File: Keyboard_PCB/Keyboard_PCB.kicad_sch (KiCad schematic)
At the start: 59 parts, among them J2 Battery, J3 JTAG, J4 EBUS, SW71 BTN, SW72 BTN, U1 STM32H7B0VBTx, U3 AP7343, U4 M95P32, Y1 25MHz, Y2 32.768 KHz

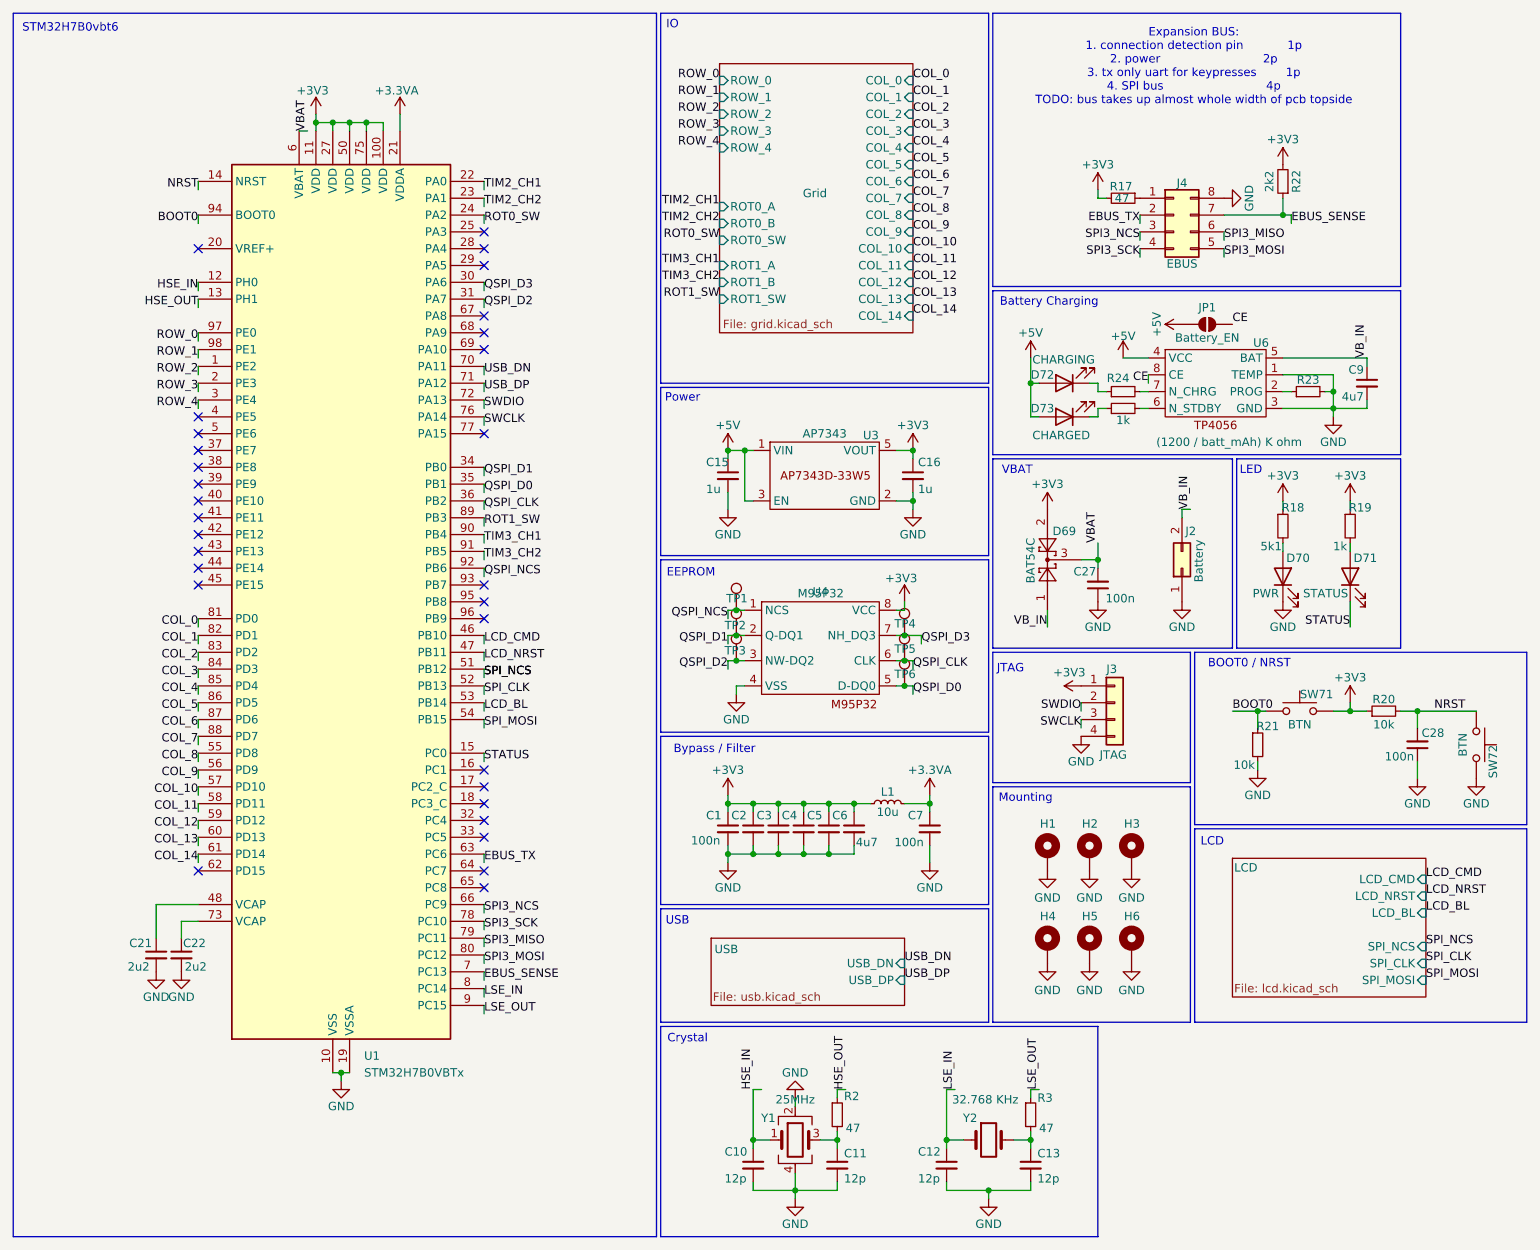
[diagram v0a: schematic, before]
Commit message: Cleaned up project
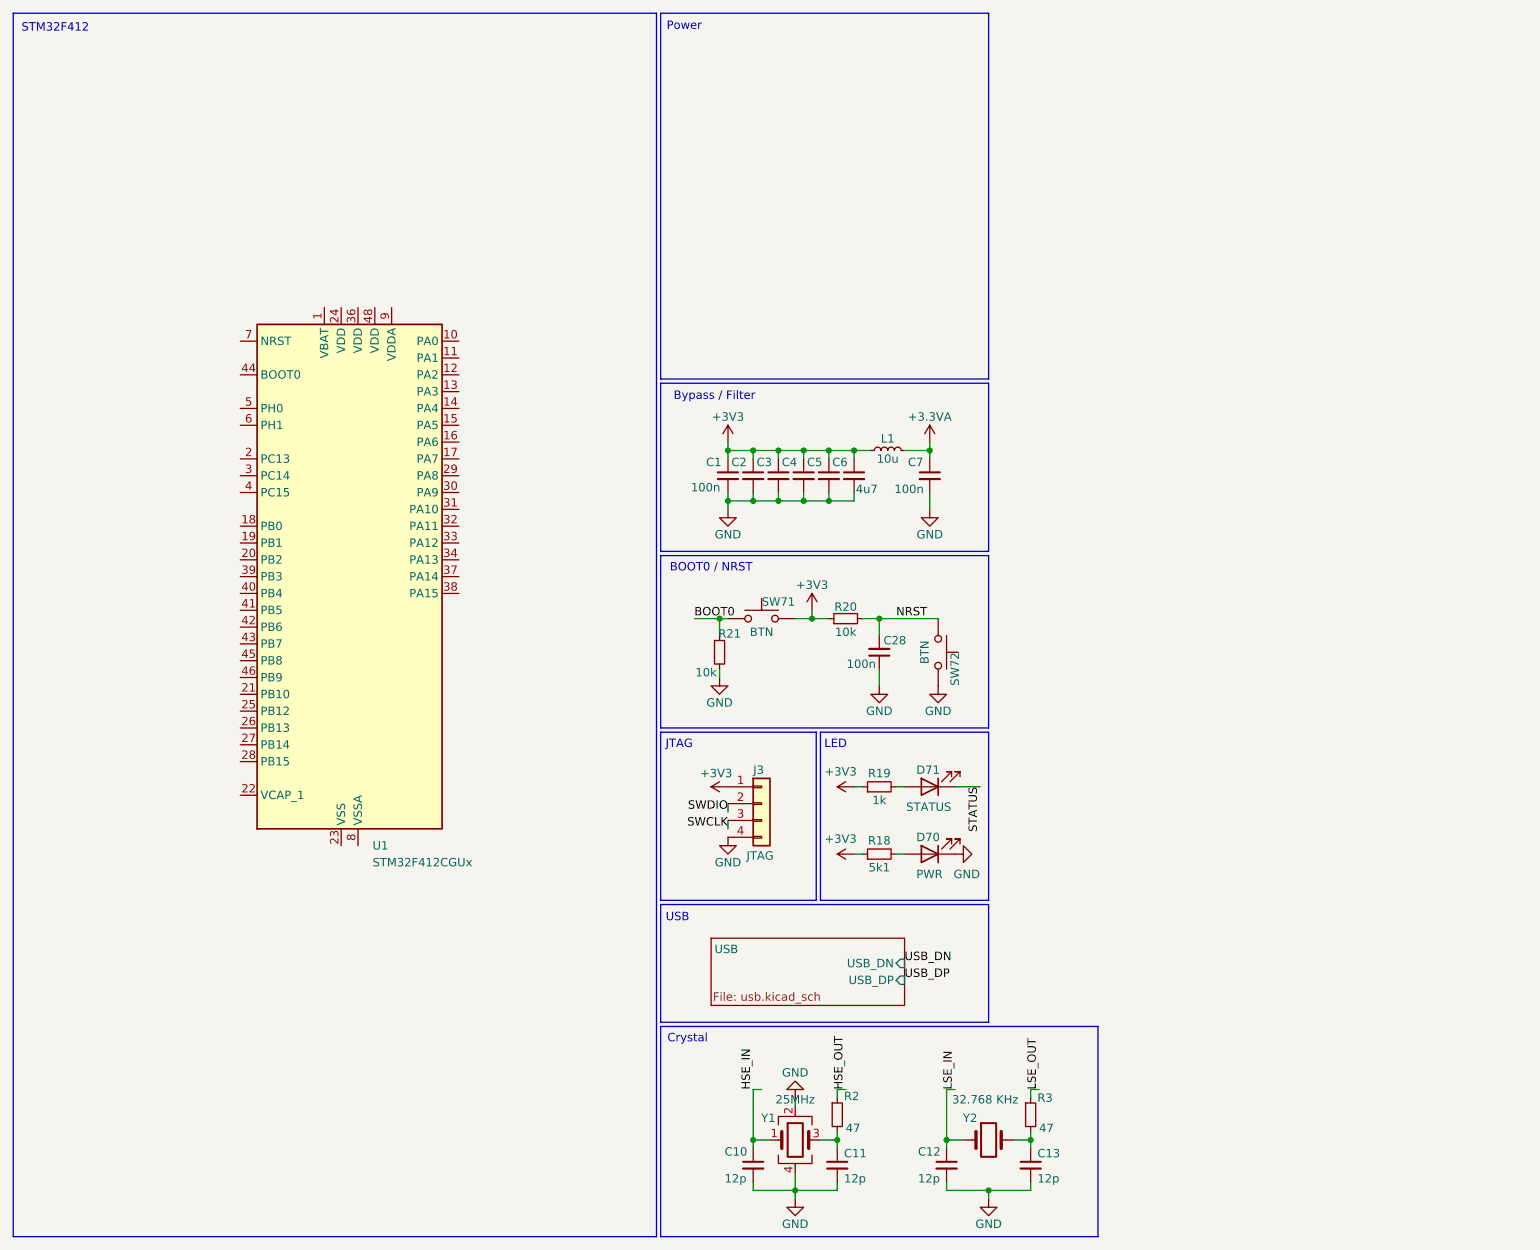
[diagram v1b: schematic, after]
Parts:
- removed C15, C16: 1u, Capacitor_SMD:C_0603_1608Metric, symbol Device:C_Small
- removed C21, C22: 2u2, Capacitor_SMD:C_0603_1608Metric, symbol Device:C_Small
- removed C27: 100n, Capacitor_SMD:C_0603_1608Metric, symbol Device:C_Small
- removed C9: 4u7, Capacitor_SMD:C_0603_1608Metric, symbol Device:C_Small
- removed D69: BAT54C, Package_TO_SOT_SMD:SOT-23, symbol Diode:BAT54C
- removed D72: CHARGING, LED_SMD:LED_0603_1608Metric, symbol Device:LED
- removed D73: CHARGED, LED_SMD:LED_0603_1608Metric, symbol Device:LED
- removed H1, H2, H3, H4, H5, H6: MountingHole_Pad, MountingHole:MountingHole_2.2mm_M2_DIN965_Pad, symbol Mechanical:MountingHole_Pad
- removed J2: Battery, Connector_PinHeader_2.00mm:PinHeader_1x02_P2.00mm_Vertical, symbol Connector_Generic:Conn_02x01
- removed J4: EBUS, Connector_PinHeader_2.00mm:PinHeader_2x04_P2.00mm_Vertical, symbol Connector_Generic:Conn_02x04_Counter_Clockwise
- removed JP1: Battery_EN, Jumper:SolderJumper-2_P1.3mm_Open_TrianglePad1.0x1.5mm, symbol Jumper:SolderJumper_2_Open
- removed R17: 47, Resistor_SMD:R_0603_1608Metric, symbol Device:R_Small
- removed R22: 2k2, Resistor_SMD:R_0603_1608Metric, symbol Device:R_Small
- removed R23: (1200 / batt_mAh) K ohm, Resistor_SMD:R_0603_1608Metric, symbol Device:R_Small
- removed R24, R25: 1k, Resistor_SMD:R_0603_1608Metric, symbol Device:R_Small
- removed TP1, TP2, TP3, TP4, TP5, TP6: TestPoint, TestPoint:TestPoint_THTPad_D2.0mm_Drill1.0mm, symbol Connector:TestPoint
- removed U1: STM32H7B0VBTx, Package_QFP:LQFP-100_14x14mm_P0.5mm, symbol MCU_ST_STM32H7:STM32H7B0VBTx
- removed U3: AP7343, Custom:SOT-25, symbol Marijn:AP7343
- removed U4: M95P32, Package_SO:PowerIntegrations_SO-8, symbol Marijn:M95P32
- removed U6: ~, Package_SO:MSOP-8_3x3mm_P0.65mm, symbol Marijn:TP4056
- added U1: STM32F412CGUx, Package_DFN_QFN:QFN-48-1EP_7x7mm_P0.5mm_EP5.6x5.6mm, symbol MCU_ST_STM32F4:STM32F412CGUx
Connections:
- new net: U1.23 (VSS), U1.35 (VSS), U1.47 (VSS), U1.49 (VSS)
- no-connect marks 30 -> 0
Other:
- removed sheet Grid
- removed sheet LCD
- note added: "STM32F412"
- note removed: "Battery Charging"
- note removed: "EEPROM"
- note removed: "Expansion BUS: 1. connection detection pin 1p 2. power 2p 3. tx only uart for keypresses 1p 4. SPI bus 4p TODO: bus takes up almost whole width of pcb topside"
- note removed: "IO"
- note removed: "LCD"
- note removed: "Mounting"
- note removed: "STM32H7B0vbt6"
- note removed: "VBAT"
- moved on the sheet: C1, C2, C28, C3, C4, C5, C6, C7, D70, D71, J3, L1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
